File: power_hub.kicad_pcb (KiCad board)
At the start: 2 copper layers, 86 x 54 mm, 51 parts, among them Q1 2N7002, Q3 SM4185, Q4 2N7002, Q5 2N7002, Q6 SM4185, Q8 SM4185

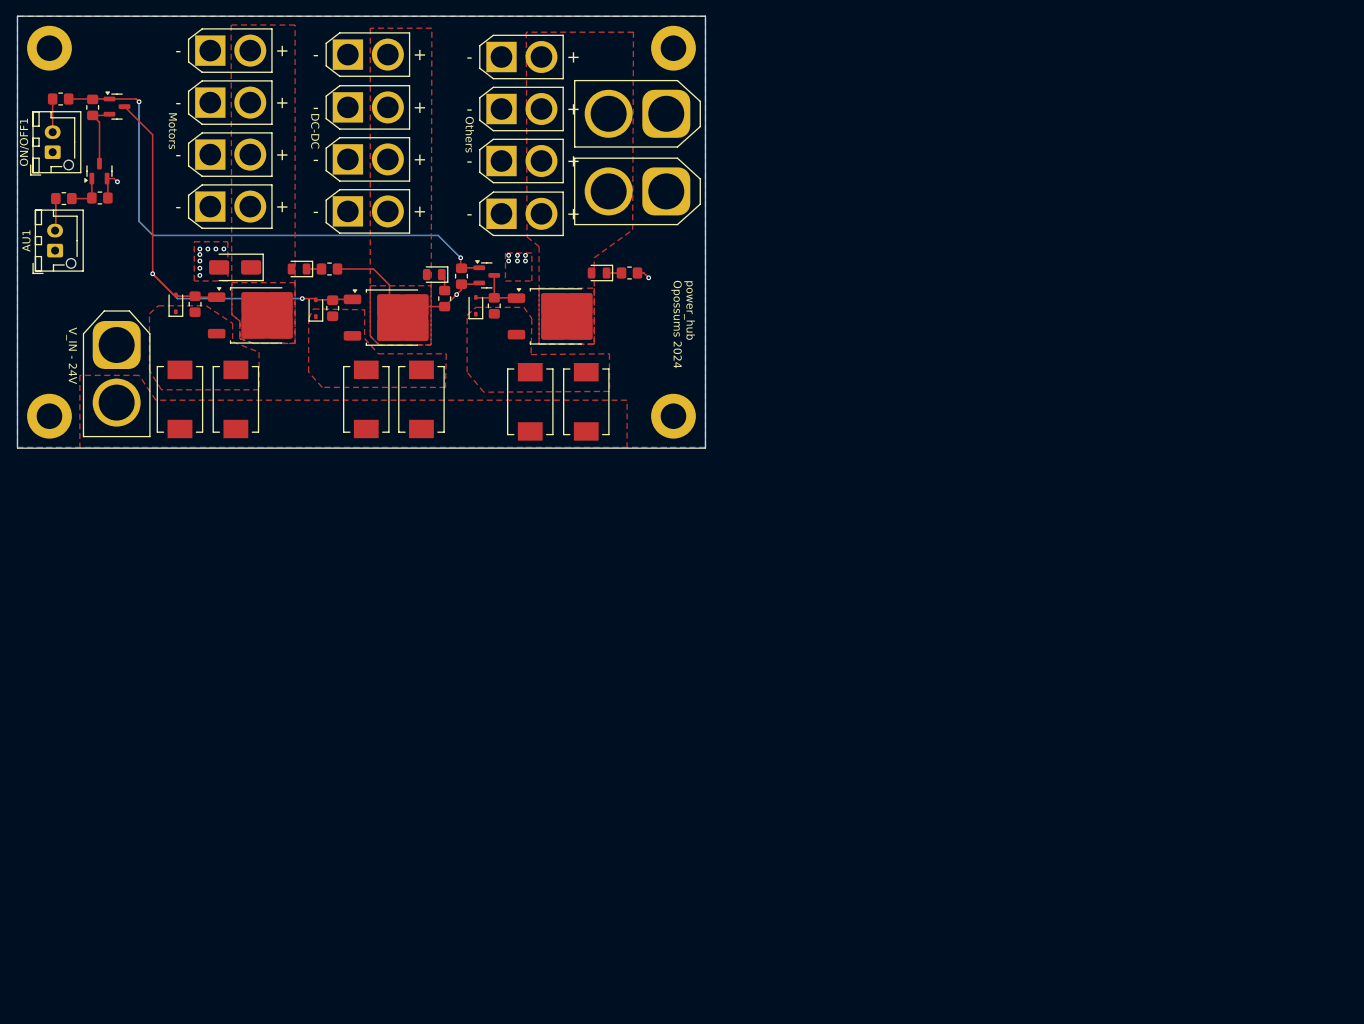
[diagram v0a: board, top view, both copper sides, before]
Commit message: update all
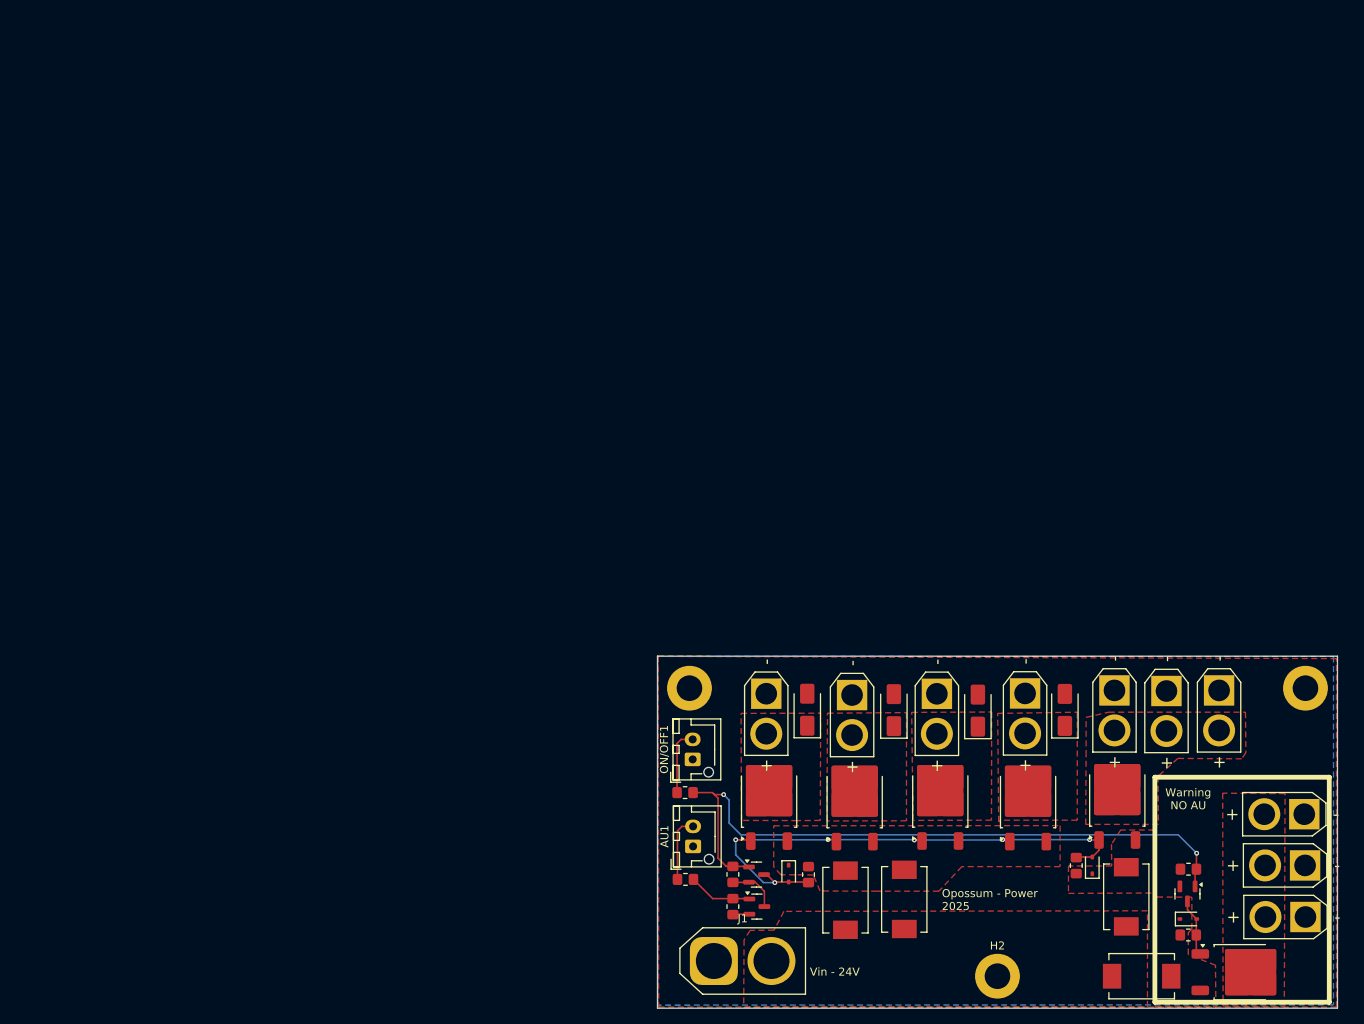
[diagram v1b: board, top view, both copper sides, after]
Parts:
- removed F10, F7: SMD1812-150C-33V 1812_SERI, Fuse:Fuse_Bourns_MF-SM_7.98x5.44mm
- removed H1: MountingHole_Pad, MountingHole:MountingHole_3.2mm_M3_DIN965_Pad
- removed LED1, LED2, LED3: GREEN, LED_SMD:LED_0805_2012Metric
- removed R13, R2, R7: 5.1k, Resistor_SMD:R_0805_2012Metric_Pad1.20x1.40mm_HandSolder
- removed xt30-female4, xt30-motor8: Conn_01x02_Pin, Connector_AMASS:AMASS_XT30U-F_1x02_P5.0mm_Vertical
- removed xt60-female1, xt60-female2, xt60-female3: Conn_01x02_Pin, Connector_AMASS:AMASS_XT60-M_1x02_P7.20mm_Vertical
- added D1: D, Diode_SMD:D_SMA, F.Cu at (129.6, 106.7)
- added D6: D, Diode_SMD:D_SMA, F.Cu at (140.1, 106.8)
- added D7: D, Diode_SMD:D_SMA, F.Cu at (118.7, 106.7)
- added J1: Conn_01x02_Pin, Connector_AMASS:AMASS_XT60-M_1x02_P7.20mm_Vertical, F.Cu at (107.0, 138.1)
- added Q2: SM4185, Package_TO_SOT_SMD:TO-252-2, F.Cu at (124.7, 118.1)
- added Q7: SM4185, Package_TO_SOT_SMD:TO-252-2, F.Cu at (135.3, 118.1)
- added Q9: SM4185, Package_TO_SOT_SMD:TO-252-2, F.Cu at (114.0, 118.1)
- moved xt30-female1 147.2 mm to (181.0, 132.6), turned to 180 degrees
- moved xt30-female2 133.6 mm to (180.9, 126.2), turned to 180 degrees
- moved xt30-female3 133.6 mm to (180.8, 119.8), turned to 180 degrees
- moved xt30-motor5 129.6 mm to (163.6, 104.3), turned to -90 degrees
- moved xt30-motor7 127.5 mm to (170.2, 104.3), turned to -90 degrees
- moved Q4 124.9 mm to (112.4, 127.3)
- moved R4 124.9 mm to (109.4, 127.3)
- moved Q5 123.3 mm to (112.4, 131.3), turned to 0 degrees
- moved H2 122.9 mm to (142.5, 140.0)
- moved xt30-motor6 120.4 mm to (157.1, 104.3), turned to -90 degrees
- moved D5 119.5 mm to (154.3, 126.2)
- moved R3 118.8 mm to (109.4, 131.3), turned to -90 degrees
- moved xt30-motor1 118.6 mm to (145.9, 104.7), turned to -90 degrees
- moved Q6 118.4 mm to (172.9, 139.5)
- moved D3 117.6 mm to (150.9, 106.7), turned to 90 degrees
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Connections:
- AU1 pad 1: Vbat_1 -> GND
- D3 pad 1: V_moteurs -> V_moteurs_1
- D3 pad 2: Vbat_1 -> GND
- H2 pad 1: Vbat_1 -> GND
- H3 pad 1: Vbat_1 -> GND
- H4 pad 1: Vbat_1 -> GND
- ON/OFF1 pad 1: Vbat_1 -> GND
- Q1 pad 2: Vbat_1 -> GND
- Q3 pad 2: V_moteurs -> V_moteurs_1
- Q5 pad 2: Vbat_1 -> GND
- Q6 pad 2: Vbat_1 -> Vbat_2
- R3 pad 2: Vbat_1 -> GND
- R5 pad 2: Vbat_1 -> GND
- xt30-female1 pad 1: Vbat_1 -> GND
- xt30-female1 pad 2: Vbat_1 -> Vbat_2
- xt30-female2 pad 1: Vbat_1 -> GND
- xt30-female2 pad 2: Vbat_1 -> Vbat_2
- xt30-female3 pad 1: Vbat_1 -> GND
- xt30-female3 pad 2: Vbat_1 -> Vbat_2
- xt30-motor1 pad 1: Vbat_1 -> GND
- xt30-motor1 pad 2: V_moteurs -> V_moteurs_1
- xt30-motor2 pad 1: Vbat_1 -> GND
- xt30-motor2 pad 2: V_moteurs -> V_moteurs_2
- xt30-motor3 pad 1: Vbat_1 -> GND
- xt30-motor3 pad 2: V_moteurs -> V_moteurs_3
- xt30-motor4 pad 1: Vbat_1 -> GND
- xt30-motor4 pad 2: V_moteurs -> V_moteurs_4
- xt30-motor5 pad 1: Vbat_1 -> GND
- xt30-motor6 pad 1: Vbat_1 -> GND
- xt30-motor7 pad 1: Vbat_1 -> GND
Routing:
- net Vbat_1: track 25.0 -> 0.00 mm, vias 17 -> 0
- net ON/OFF: track 69.6 -> 84.6 mm
- net /on/off/au: track 58.0 -> 69.8 mm, vias 2 -> 6
- net Net-(AU1-Pin_2): track 4.04 -> 8.25 mm
- net Net-(ON/OFF1-Pin_2): track 4.15 -> 8.31 mm
- net AU: track 4.96 -> 8.00 mm
- net Net-(Q4-S): track 8.54 -> 6.33 mm
- net Net-(LED1-K): track 2.15 -> 0.00 mm
- net GND: track 0.00 -> 2.08 mm
- net Net-(LED3-K): track 2.00 -> 0.00 mm
- net Net-(LED2-K): track 1.86 -> 0.00 mm
- net Net-(D4-A): track 7.91 -> 7.27 mm
- added copper zone on B.Cu, net GND
- added copper zone on F.Cu, net GND
- added copper zone on F.Cu, net V_moteurs_1
- added copper zone on F.Cu, net V_moteurs_2
- added copper zone on F.Cu, net V_moteurs_3
- added copper zone on F.Cu, net V_moteurs_4
- added copper zone on F.Cu, net Vbat_2
- removed copper zone on F.Cu, net V_moteurs
- removed copper zone on B.Cu, net Vbat_1
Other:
- board size 86 x 54 mm -> 85 x 44 mm
- board text added: "Opossum - Power 2025"
- board text added: "Vin - 24V"
- board text added: "Warning NO AU"
- board text removed: "DC-DC"
- board text removed: "Motors"
- board text removed: "Others"
- board text removed: "V_IN - 24V"
- board text removed: "power_hub Opossums 2024"
